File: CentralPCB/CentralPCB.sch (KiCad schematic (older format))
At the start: 60 parts, among them J1 POWER HEADER, J2 SPI Header, J3 Conn_01x24, J4 Conn_01x24, J5 Conn_02x16_Odd_Even, J6 Conn_Coaxial, J7 Conn_02x10_Odd_Even, J8 Conn_01x05, U1 AD8531, U2 Teensy4.1, U3 BA7810CP-E2

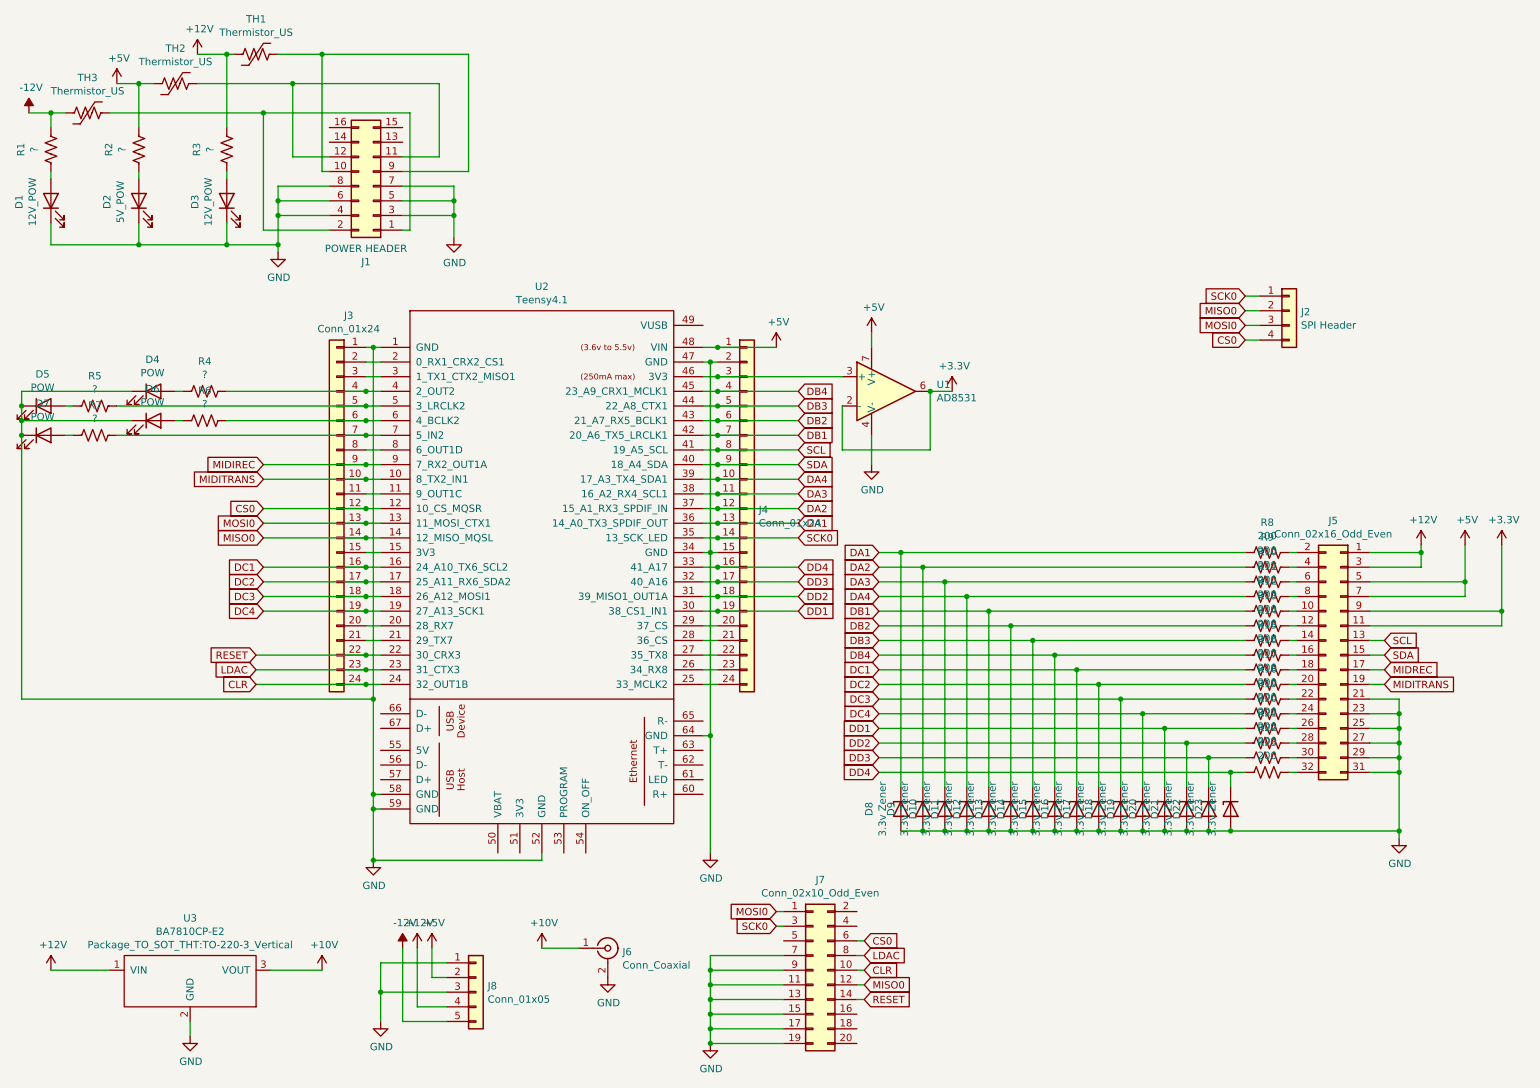
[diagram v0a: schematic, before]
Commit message: Revert "Sav"
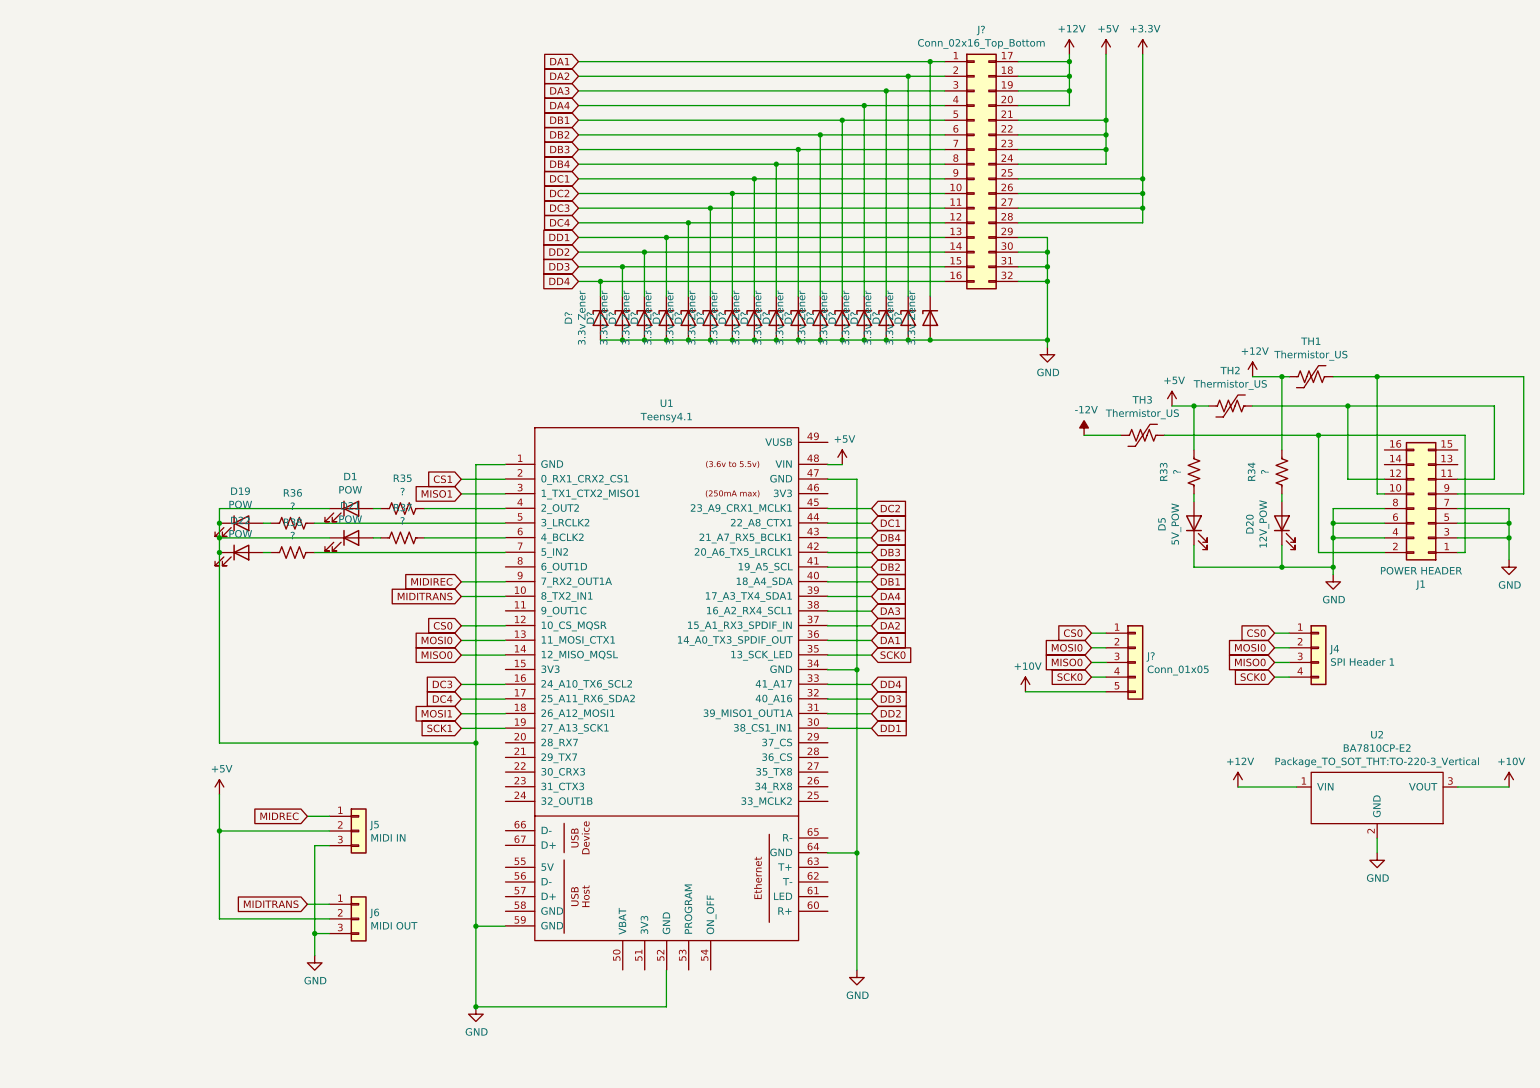
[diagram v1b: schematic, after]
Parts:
- removed D1: 12V_POW, LED_THT:LED_D3.0mm, symbol Device:LED
- removed J3, J4: Conn_01x24, Connector_PinSocket_2.54mm:PinSocket_1x24_P2.54mm_Vertical, symbol Connector_Generic:Conn_01x24
- removed J5: Conn_02x16_Odd_Even, Connector_PinSocket_2.54mm:PinSocket_2x16_P2.54mm_Vertical, symbol Connector_Generic:Conn_02x16_Odd_Even
- removed J6: Conn_Coaxial, Connector_Coaxial:SMB_Jack_Vertical, symbol Connector:Conn_Coaxial
- removed J7: Conn_02x10_Odd_Even, Connector_PinSocket_2.54mm:PinSocket_2x10_P2.54mm_Vertical, symbol Connector_Generic:Conn_02x10_Odd_Even
- removed J8: Conn_01x05, Connectors_Phoenix:PhoenixContact_GMSTBVA-G_05x7.50mm_Vertical, symbol Connector_Generic:Conn_01x05
- removed R1: ?, Resistor_SMD:R_0805_2012Metric, symbol Device:R_US
- removed R10, R11, R12, R13, R14, R15, R16, R17, R18, R19, R20, R21, R22, R23, R8, R9: 200, Resistor_SMD:R_0805_2012Metric, symbol Device:R_US
- removed U1: AD8531, Package_SO:SOIC-8_3.9x4.9mm_P1.27mm, symbol Amplifier_Operational:OP179GS
- removed U2: Teensy4.1, teensy:Teensy41, symbol teensy:Teensy4.1
- added J5: MIDI IN, Connector_PinSocket_2.54mm:PinSocket_1x03_P2.54mm_Vertical, symbol Connector_Generic:Conn_01x03
- added J6: MIDI OUT, Connector_PinSocket_2.54mm:PinSocket_1x03_P2.54mm_Vertical, symbol Connector_Generic:Conn_01x03
- added J?: Conn_02x16_Top_Bottom, Connector_PinSocket_2.54mm:PinSocket_2x16_P2.54mm_Vertical, symbol Connector_Generic:Conn_02x16_Top_Bottom
- added J?: Conn_01x05, symbol Connector_Generic:Conn_01x05
- added U1: Teensy4.1, symbol teensy:Teensy4.1
- J4: renamed from J2; value SPI Header -> SPI Header 1
- renumbered D4 to D1, D5 to D19, D3 to D20, D6 to D21, D7 to D22, D2 to D5, D9 to D?, D10 to D?, D11 to D?, D12 to D?, D13 to D?, D14 to D?, D15 to D?, D16 to D?, D17 to D?, D18 to D?, D19 to D?, D20 to D?, D21 to D?, D22 to D?, D23 to D?, D8 to D?, R2 to R33, R3 to R34, R4 to R35, R5 to R36, R6 to R37, R7 to R38, U3 to U2
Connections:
- net labels added: CS1, MISO1, MOSI1, SCK1
- net labels removed: CLR, LDAC, RESET, SCL, SDA
- wire segments 309 -> 218
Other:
- moved on the sheet: D1, D19, D20, D21, D22, D5, D?, J1, J4, R33, R34, R35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
